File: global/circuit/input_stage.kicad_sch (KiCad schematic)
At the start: 7 parts, among them U6 TL081H

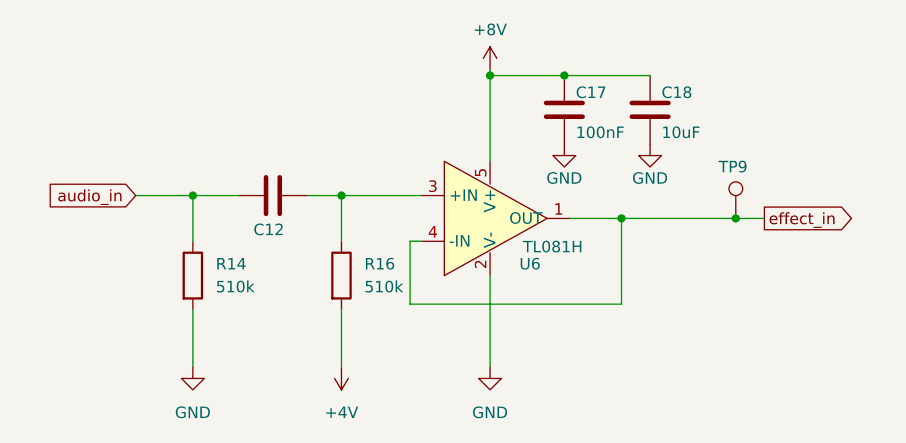
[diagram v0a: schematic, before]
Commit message: rework global circuits
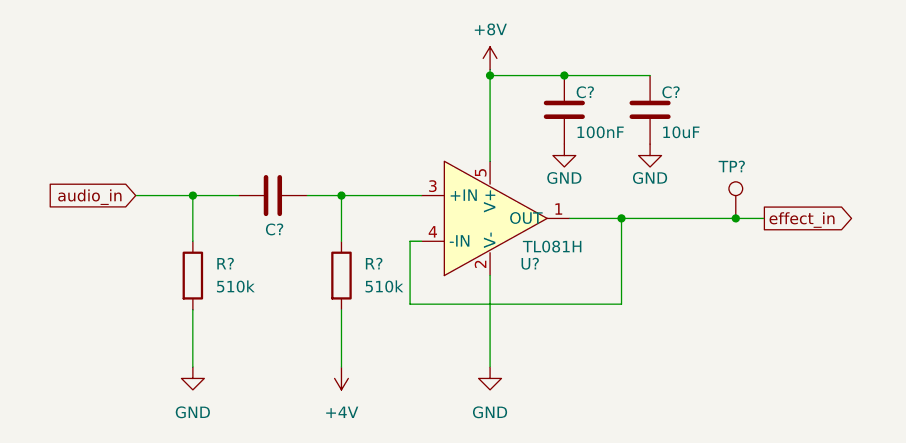
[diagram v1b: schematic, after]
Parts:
- renumbered C18 to C?, C17 to C?, C12 to C?, R16 to R?, R14 to R?, TP9 to TP?, U6 to U?
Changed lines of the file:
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@@
   (symbol (lib_id "power:+4V") (at 96.52 70.485 180) (unit 1)
     (in_bom yes) (on_board yes) (fields_autoplaced)
-    (property "Reference" "#PWR0116" (id 0) (at 96.52 66.675 0)
+    (property "Reference" "#PWR?" (id 0) (at 96.52 66.675 0)
       (effects (font (size 1.27 1.27)) hide)
     )
@@
   (symbol (lib_id "Device:C") (at 130.81 41.91 0) (unit 1)
     (in_bom yes) (on_board yes)
-    (property "Reference" "C18" (id 0) (at 132.08 40.005 0)
+    (property "Reference" "C?" (id 0) (at 132.08 40.005 0)
       (effects (font (size 1.27 1.27)) (justify left))
     )
@@
   (symbol (lib_id "Device:R") (at 96.52 60.325 0) (unit 1)
     (in_bom yes) (on_board yes) (fields_autoplaced)
-    (property "Reference" "R16" (id 0) (at 99.06 59.0549 0)
+    (property "Reference" "R?" (id 0) (at 99.06 59.0549 0)
       (effects (font (size 1.27 1.27)) (justify left))
     )
@@
   (symbol (lib_id "power:GND") (at 121.285 45.72 0) (unit 1)
     (in_bom yes) (on_board yes)
-    (property "Reference" "#PWR034" (id 0) (at 121.285 52.07 0)
+    (property "Reference" "#PWR?" (id 0) (at 121.285 52.07 0)
       (effects (font (size 1.27 1.27)) hide)
     )
@@
   (symbol (lib_id "Amplifier_Operational:TL081H") (at 113.03 53.975 0) (unit 1)
     (in_bom yes) (on_board yes)
-    (property "Reference" "U6" (id 0) (at 117.475 59.055 0))
+    (property "Reference" "U?" (id 0) (at 117.475 59.055 0))
     (property "Value" "TL081H" (id 1) (at 120.015 57.15 0))
     (property "Footprint" "Package_TO_SOT_SMD:SOT-23-5_HandSoldering" (id 2) (at 113.03 53.975 0)
@@
   (symbol (lib_id "power:GND") (at 80.01 70.485 0) (unit 1)
     (in_bom yes) (on_board yes) (fields_autoplaced)
-    (property "Reference" "#PWR029" (id 0) (at 80.01 76.835 0)
+    (property "Reference" "#PWR?" (id 0) (at 80.01 76.835 0)
       (effects (font (size 1.27 1.27)) hide)
     )
@@
   (symbol (lib_id "power:+8V") (at 113.03 37.465 0) (unit 1)
     (in_bom yes) (on_board yes)
-    (property "Reference" "#PWR032" (id 0) (at 113.03 41.275 0)
+    (property "Reference" "#PWR?" (id 0) (at 113.03 41.275 0)
       (effects (font (size 1.27 1.27)) hide)
     )
@@
   (symbol (lib_id "Connector:TestPoint") (at 140.335 53.975 0) (unit 1)
     (in_bom yes) (on_board yes)
-    (property "Reference" "TP9" (id 0) (at 138.43 48.26 0)
+    (property "Reference" "TP?" (id 0) (at 138.43 48.26 0)
       (effects (font (size 1.27 1.27)) (justify left))
     )
@@
   (symbol (lib_id "power:GND") (at 130.81 45.72 0) (unit 1)
     (in_bom yes) (on_board yes)
-    (property "Reference" "#PWR035" (id 0) (at 130.81 52.07 0)
+    (property "Reference" "#PWR?" (id 0) (at 130.81 52.07 0)
       (effects (font (size 1.27 1.27)) hide)
     )
@@
   (symbol (lib_id "Device:R") (at 80.01 60.325 0) (unit 1)
     (in_bom yes) (on_board yes) (fields_autoplaced)
-    (property "Reference" "R14" (id 0) (at 82.55 59.0549 0)
+    (property "Reference" "R?" (id 0) (at 82.55 59.0549 0)
       (effects (font (size 1.27 1.27)) (justify left))
     )
@@
   (symbol (lib_id "Device:C") (at 121.285 41.91 0) (unit 1)
     (in_bom yes) (on_board yes)
-    (property "Reference" "C17" (id 0) (at 122.555 40.005 0)
+    (property "Reference" "C?" (id 0) (at 122.555 40.005 0)
       (effects (font (size 1.27 1.27)) (justify left))
     )
@@
   (symbol (lib_id "power:GND") (at 113.03 70.485 0) (unit 1)
     (in_bom yes) (on_board yes) (fields_autoplaced)
-    (property "Reference" "#PWR033" (id 0) (at 113.03 76.835 0)
+    (property "Reference" "#PWR?" (id 0) (at 113.03 76.835 0)
       (effects (font (size 1.27 1.27)) hide)
     )
@@
   (symbol (lib_id "Device:C") (at 88.9 51.435 90) (unit 1)
     (in_bom yes) (on_board yes)
-    (property "Reference" "C12" (id 0) (at 90.17 55.245 90)
+    (property "Reference" "C?" (id 0) (at 90.17 55.245 90)
       (effects (font (size 1.27 1.27)) (justify left))
     )
